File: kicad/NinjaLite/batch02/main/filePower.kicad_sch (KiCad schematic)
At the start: 38 parts, among them J1 ALI_USB, J2 Barrel_Jack_Switch, Q1 Q_NMOS_GSD, U11 IP2721, U12 TPS63710DRRR, U14 TCR3DF33,LM(CT, U3 BD433M5FP-CE2, U6 BA178M05FP-E2

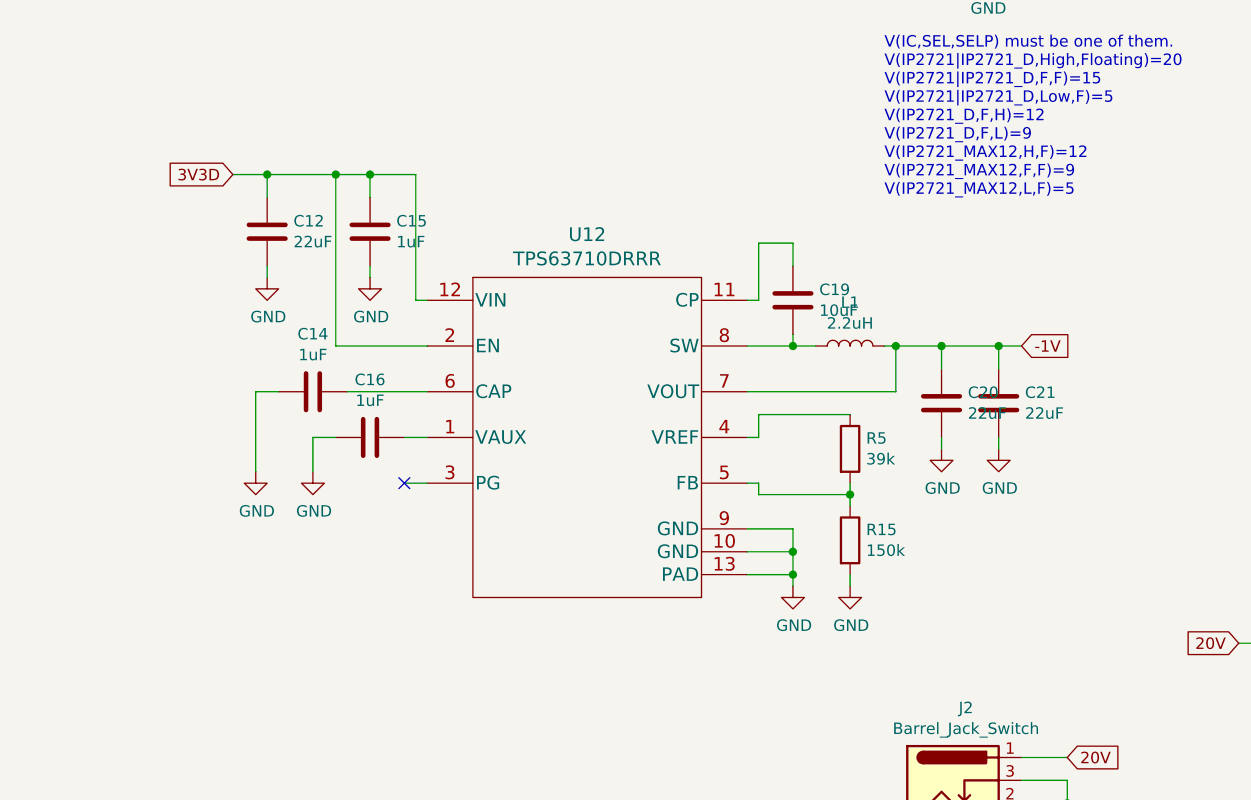
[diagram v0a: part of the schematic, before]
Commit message: sync
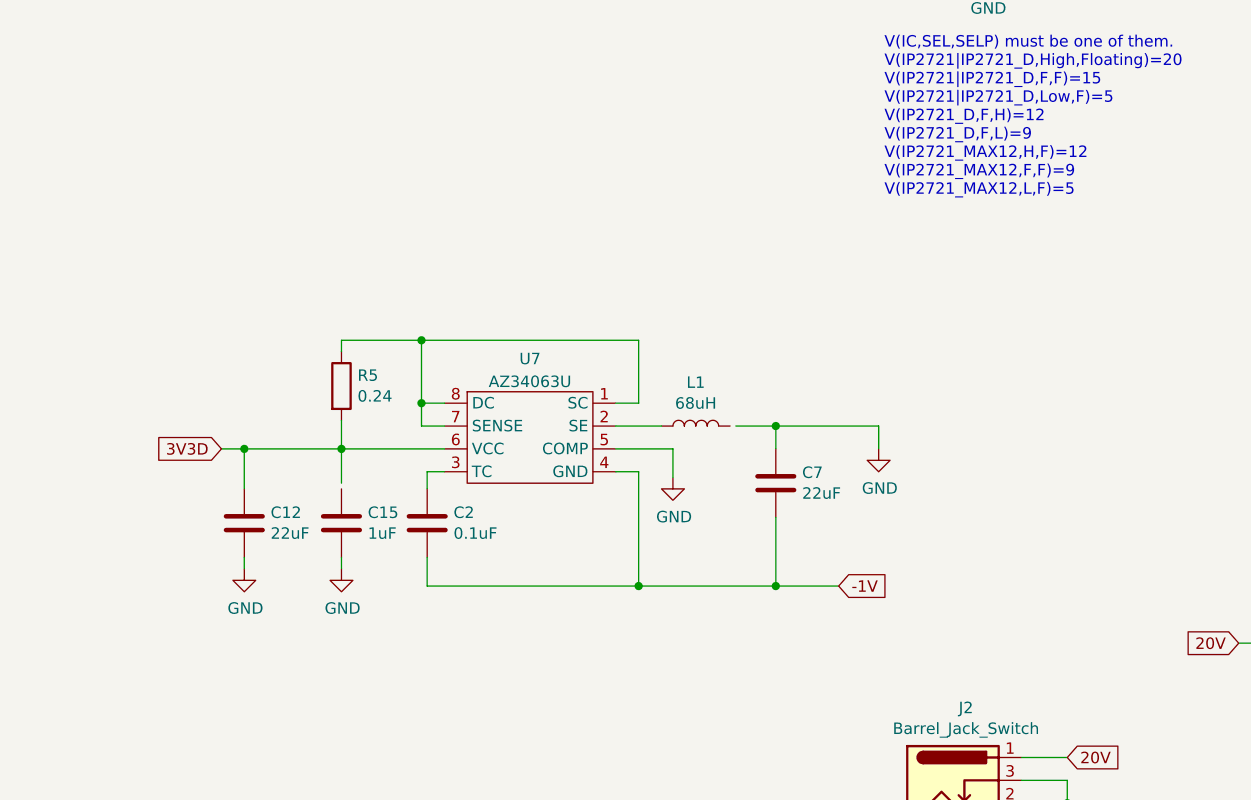
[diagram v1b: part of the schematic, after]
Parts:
- removed C14, C16: 1uF, Capacitor_SMD:C_0603_1608Metric, symbol Device:C
- removed C19: 10uF, Capacitor_SMD:C_0805_2012Metric, symbol Device:C
- removed C20, C21: 22uF, Capacitor_SMD:C_1210_3225Metric, symbol Device:C
- removed R15: 150k, Resistor_SMD:R_0603_1608Metric, symbol Device:R
- removed U12: TPS63710DRRR, Ninja-qPCR:TPS63710DRRR, symbol Ninja-qPCR:TPS63710DRRR
- added C2: 0.1uF, Capacitor_SMD:C_0603_1608Metric, symbol Device:C
- added C7: 22uF, Capacitor_SMD:C_1210_3225Metric, symbol Device:C
- added U7: AZ34063U, Package_SO:SOP-8_3.9x4.9mm_P1.27mm, symbol Ninja-qPCR:AZ34063U
- L1: value 2.2uH -> 68uH; footprint Capacitor_SMD:C_0805_2012Metric -> (none)
- R5: value 39k -> 0.24
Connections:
- net -1V: now also C2.2, C7.2, U7.4 (GND); no longer L1.2
- net 3V3D: now also R5.2, U7.6 (VCC); no longer C15.1
- net GND: now also C7.1, U7.5 (COMP)
- net at R5.1: now also U7.1 (SC), U7.7 (SENSE), U7.8 (DC)
- net at L1.1: now also U7.2 (SE)
- new net: C2.1, U7.3 (TC)
- no-connect marks 2 -> 1
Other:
- moved on the sheet: C12, C15
